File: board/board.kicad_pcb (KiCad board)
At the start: 2 copper layers, 21 x 13 mm, 1 part

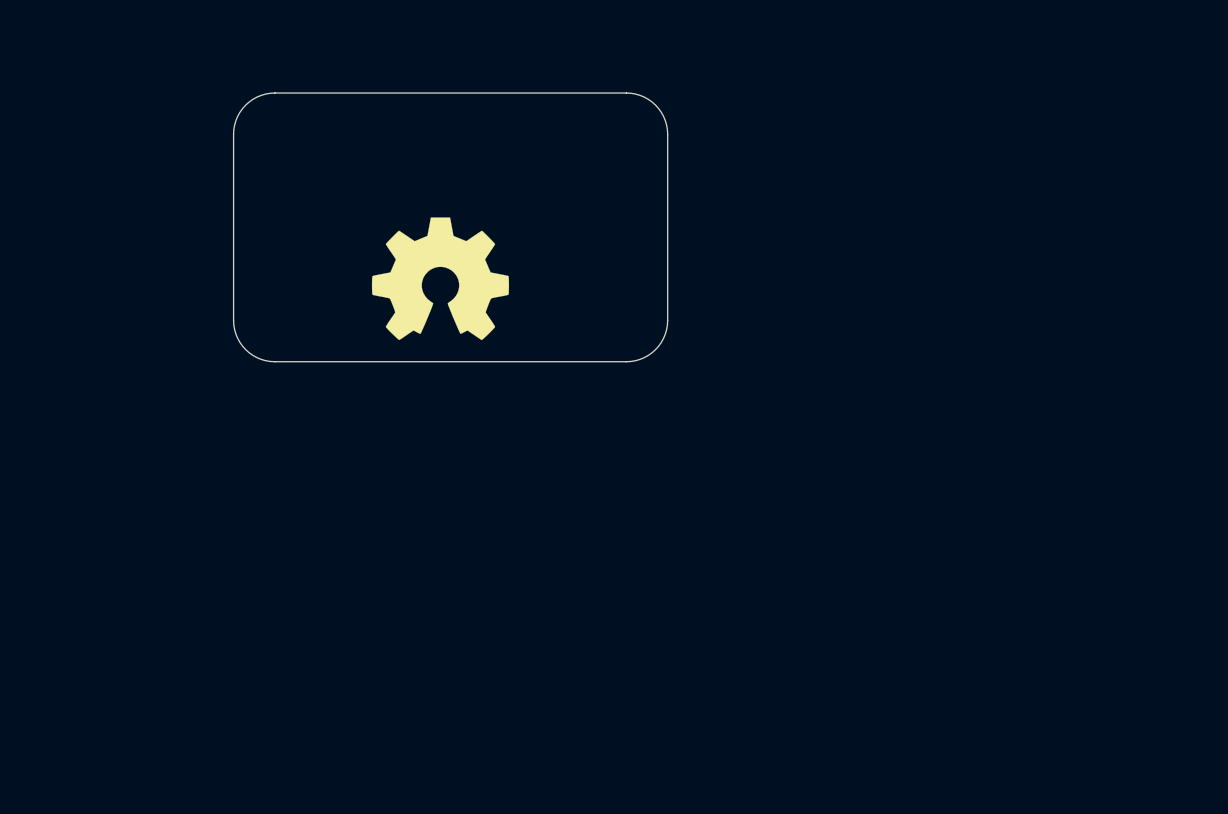
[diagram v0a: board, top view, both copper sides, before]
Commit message: initial
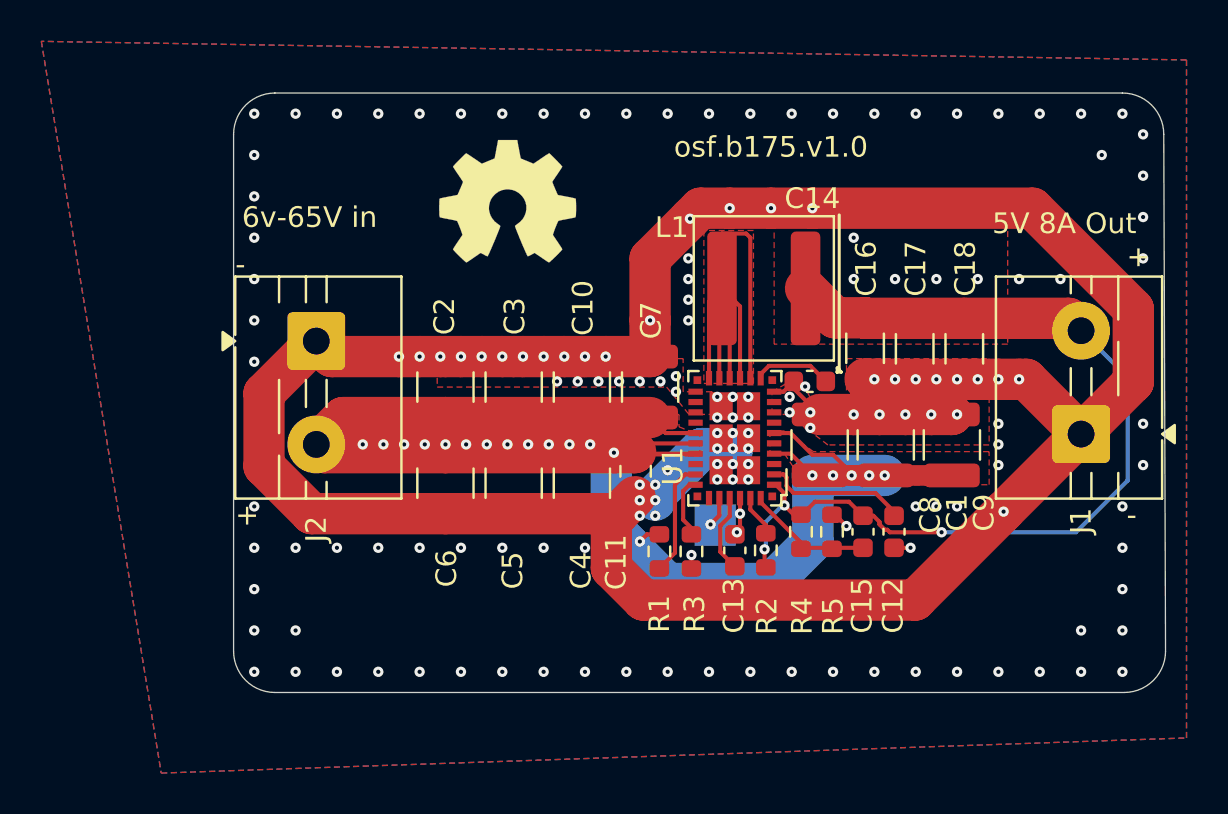
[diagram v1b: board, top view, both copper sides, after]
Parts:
- added C1: 4.7uF, Capacitor_SMD:C_1210_3225Metric, F.Cu at (171.6, 107.0)
- added C10: 4.7uF, Capacitor_SMD:C_1210_3225Metric, F.Cu at (156.8, 104.2)
- added C11: 100nF, Capacitor_SMD:C_0805_2012Metric, F.Cu at (159.4, 108.3)
- added C12: 1uF, Capacitor_SMD:C_0603_1608Metric, F.Cu at (171.9, 111.2)
- added C13: 100nF, Capacitor_SMD:C_0603_1608Metric, F.Cu at (164.2, 112.1)
- added C14: 100nF, Capacitor_SMD:C_0603_1608Metric, F.Cu at (167.9, 104.0)
- added C15: 2.2pF, Capacitor_SMD:C_0603_1608Metric, F.Cu at (170.4, 111.2)
- added C16: 100uF, Capacitor_SMD:C_1206_3216Metric, F.Cu at (170.6, 102.3)
- added C17: 10uF, Capacitor_SMD:C_1206_3216Metric, F.Cu at (172.9, 102.4)
- added C18: 1uF, Capacitor_SMD:C_1206_3216Metric, F.Cu at (175.3, 102.4)
- added C2: 4.7uF, Capacitor_SMD:C_1210_3225Metric, F.Cu at (150.2, 104.2)
- added C3: 4.7uF, Capacitor_SMD:C_1210_3225Metric, F.Cu at (153.6, 104.2)
- added C4: 4.7uF, Capacitor_SMD:C_1210_3225Metric, F.Cu at (156.8, 108.9)
- added C5: 4.7uF, Capacitor_SMD:C_1210_3225Metric, F.Cu at (153.6, 108.9)
- added C6: 4.7uF, Capacitor_SMD:C_1210_3225Metric, F.Cu at (150.2, 108.9)
- added C7: 4.7uF, Capacitor_SMD:C_1210_3225Metric, F.Cu at (160.2, 104.2)
- added C8: 4.7uF, Capacitor_SMD:C_1210_3225Metric, F.Cu at (168.3, 107.0)
- added C9: 4.7uF, Capacitor_SMD:C_1210_3225Metric, F.Cu at (174.8, 107.0)
- added J1: Conn_01x02_Socket, TerminalBlock:TerminalBlock_MaiXu_MX126-5.0-02P_1x02_P5.00mm, F.Cu at (181.0, 106.5)
- added J2: Conn_01x02_Socket, TerminalBlock:TerminalBlock_MaiXu_MX126-5.0-02P_1x02_P5.00mm, F.Cu at (144.0, 102.0)
- added L1: 1uH, Inductor_SMD:L_Coilcraft_XAL6030-XXX, F.Cu at (165.7, 99.5)
- added R1: 100k, Resistor_SMD:R_0603_1608Metric, F.Cu at (160.6, 112.2)
- added R2: 100k, Resistor_SMD:R_0603_1608Metric, F.Cu at (165.8, 112.1)
- added R3: 18k, Resistor_SMD:R_0603_1608Metric, F.Cu at (162.2, 112.2)
- added R4: 1M, Resistor_SMD:R_0603_1608Metric, F.Cu at (167.4, 111.2)
- added R5: 243k, Resistor_SMD:R_0603_1608Metric, F.Cu at (168.9, 111.2)
- added TPM1: Mode, TestPoint:TestPoint_Pad_2.0x2.0mm, B.Cu at (163.3, 110.9)
- added U1: LT8645S, b175:LQFN-32-6EP_4x6mm_P0.5mm, F.Cu at (164.2, 106.7)
- moved LOGO1 4.96 mm to (153.2, 95.2)
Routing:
- net GND: track 0.00 -> 140.9 mm, vias 0 -> 165
- net /8A_DCDC/In: track 0.00 -> 98.6 mm, vias 0 -> 19
- net /8A_DCDC/5V: track 0.00 -> 45.8 mm, vias 0 -> 3
- net /8A_DCDC/SW: track 0.00 -> 29.1 mm
- net Net-(U1-INTVCC): track 0.00 -> 6.99 mm
- net /8A_DCDC/FB: track 0.00 -> 6.21 mm
- net /8A_DCDC/En: track 0.00 -> 5.50 mm
- net Net-(U1-BST): track 0.00 -> 3.83 mm
- net Net-(U1-TR/SS): track 0.00 -> 3.78 mm
- net Net-(U1-RT): track 0.00 -> 2.99 mm
- net Net-(U1-PG): track 0.00 -> 2.06 mm
- net /8A_DCDC/Mode: track 0.00 -> 1.45 mm, vias 0 -> 1
- added copper zone on F.Cu, net /8A_DCDC/5V
- added copper zone on F.Cu, net /8A_DCDC/In
- added copper zone on F.Cu, net /8A_DCDC/SW
- added copper zone on B.Cu, net GND
- added copper zone on F.Cu, net GND
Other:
- board size 21 x 13 mm -> 45.1 x 29 mm
- board text added: "+"
- board text added: "-"
- board text added: "5V 8A Out"
- board text added: "6v-65V in"
- board text added: "osf.b175.v1.0"
